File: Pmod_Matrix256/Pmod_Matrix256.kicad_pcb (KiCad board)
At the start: 2 copper layers, 92.6 x 42.2 mm, 22 parts, among them J1 Pmod_Header, U1 OSLB56317-ARA, U2 74AHC595, U3 74AHC595, U4 74AHC595, U5 74AHC595

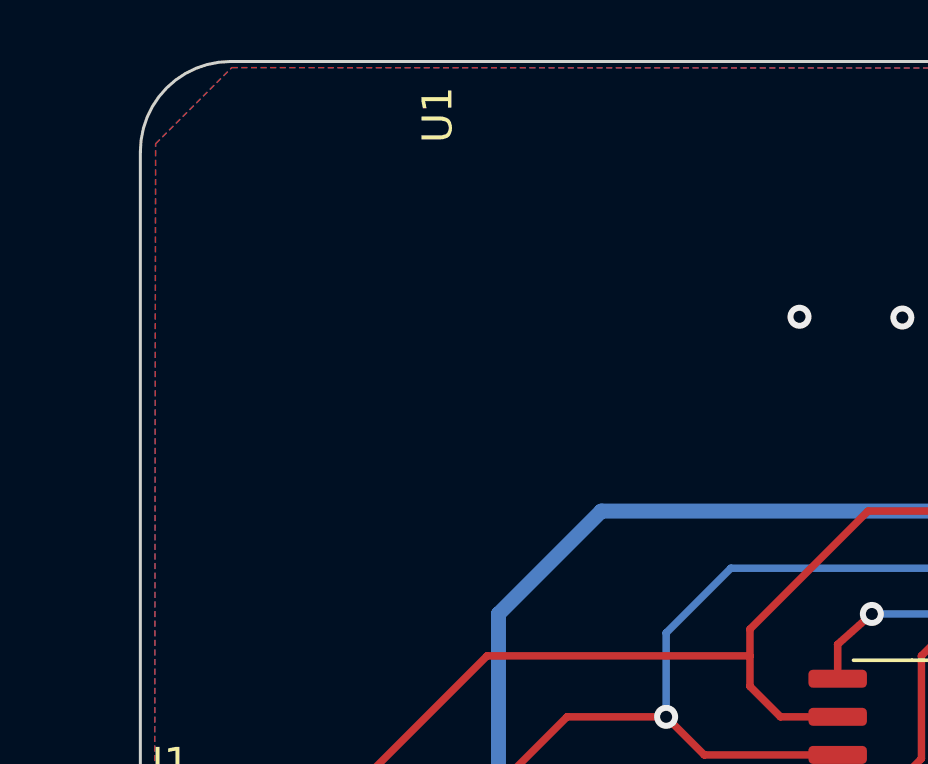
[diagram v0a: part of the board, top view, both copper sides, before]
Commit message: 0812
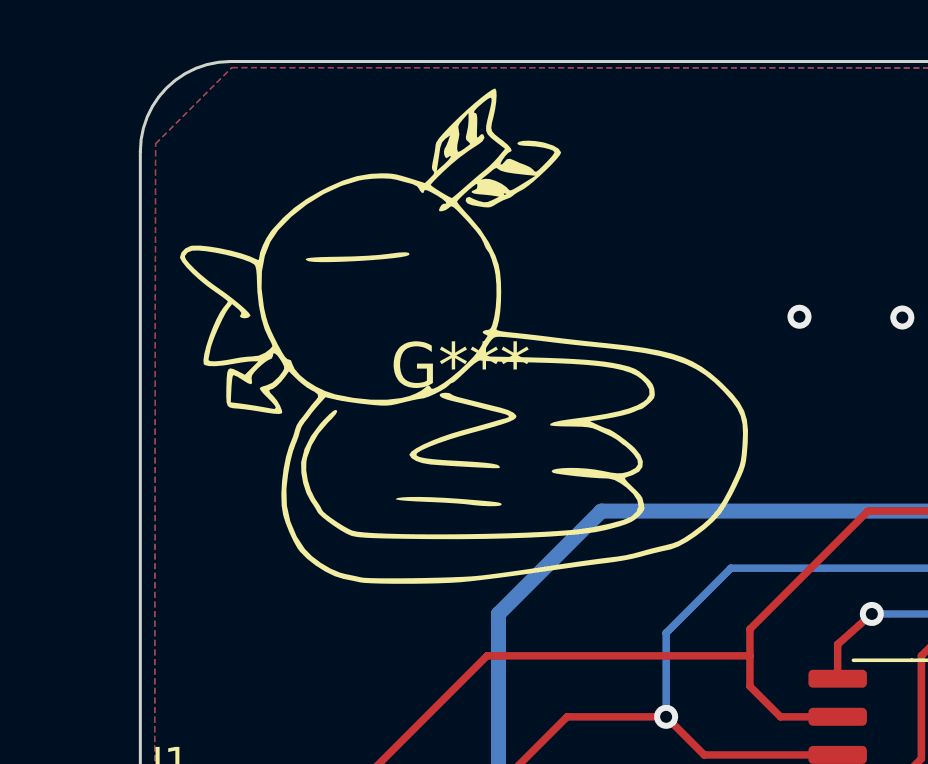
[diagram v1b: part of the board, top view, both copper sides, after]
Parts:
- added G***: LOGO, MyLibrary:kamo20, F.Cu at (104.6, 103.9)
